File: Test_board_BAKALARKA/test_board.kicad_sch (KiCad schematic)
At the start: 6 parts, among them SW1 SW_SPST, SW2 SW_SPST, U2 ESP32-S3-WROOM-2

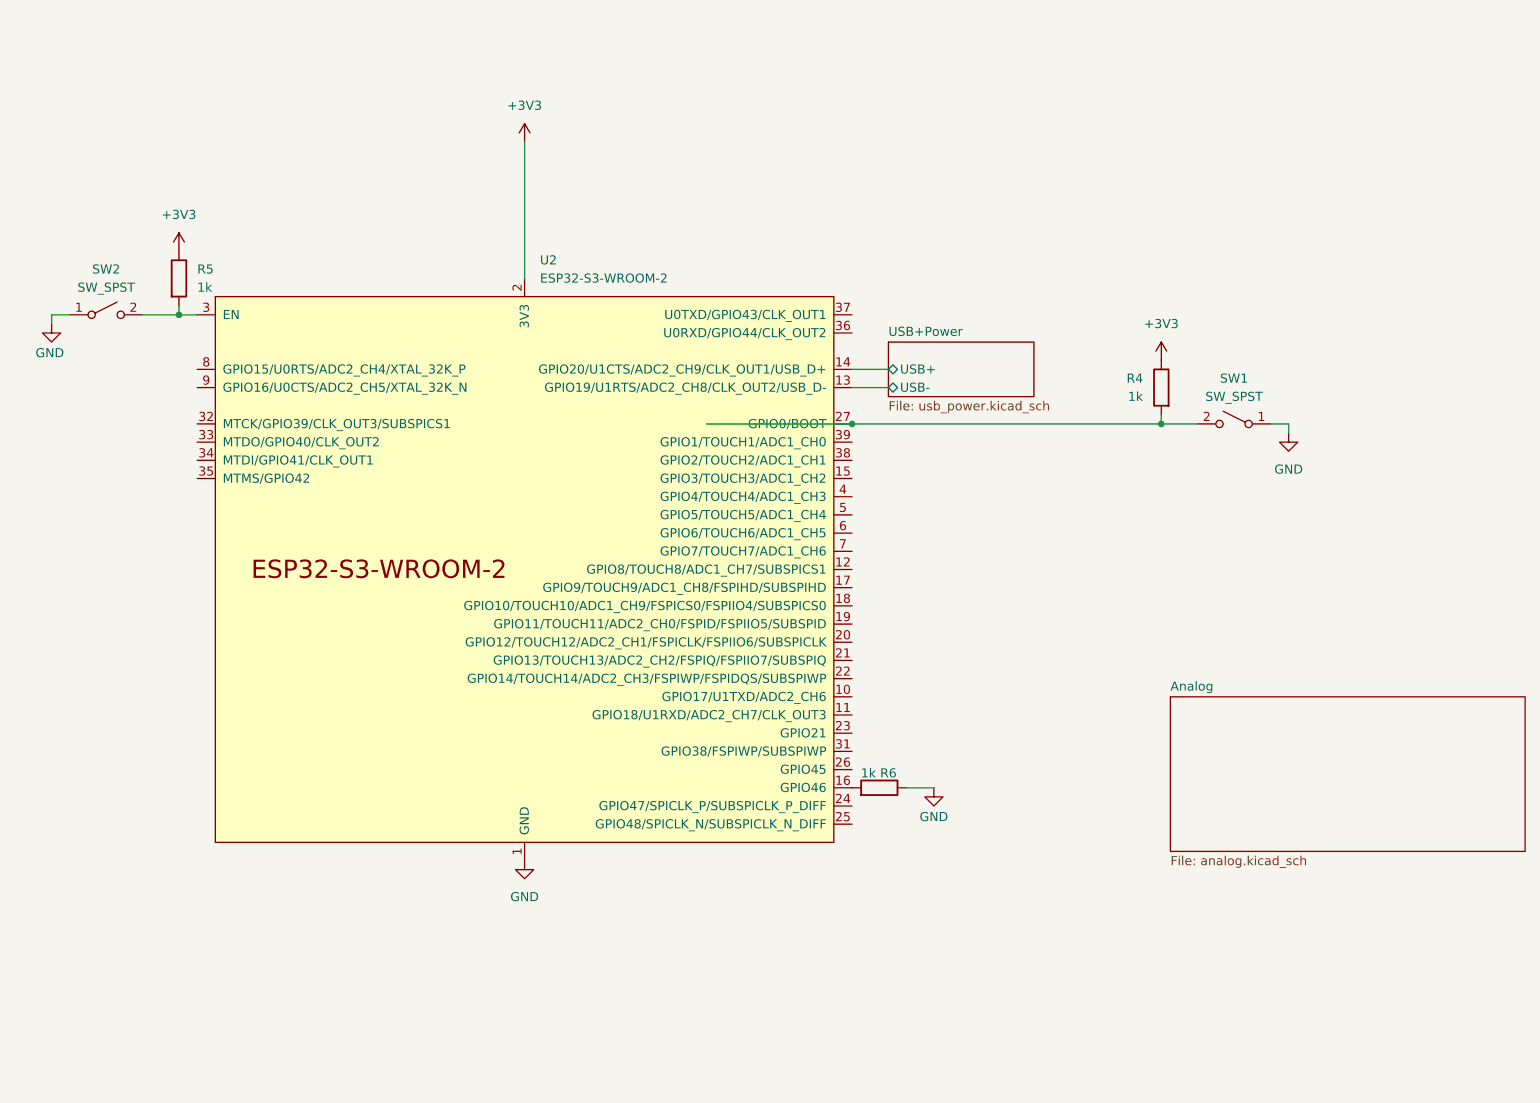
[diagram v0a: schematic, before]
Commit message: pridani textu peak detect, xor phase, signal source
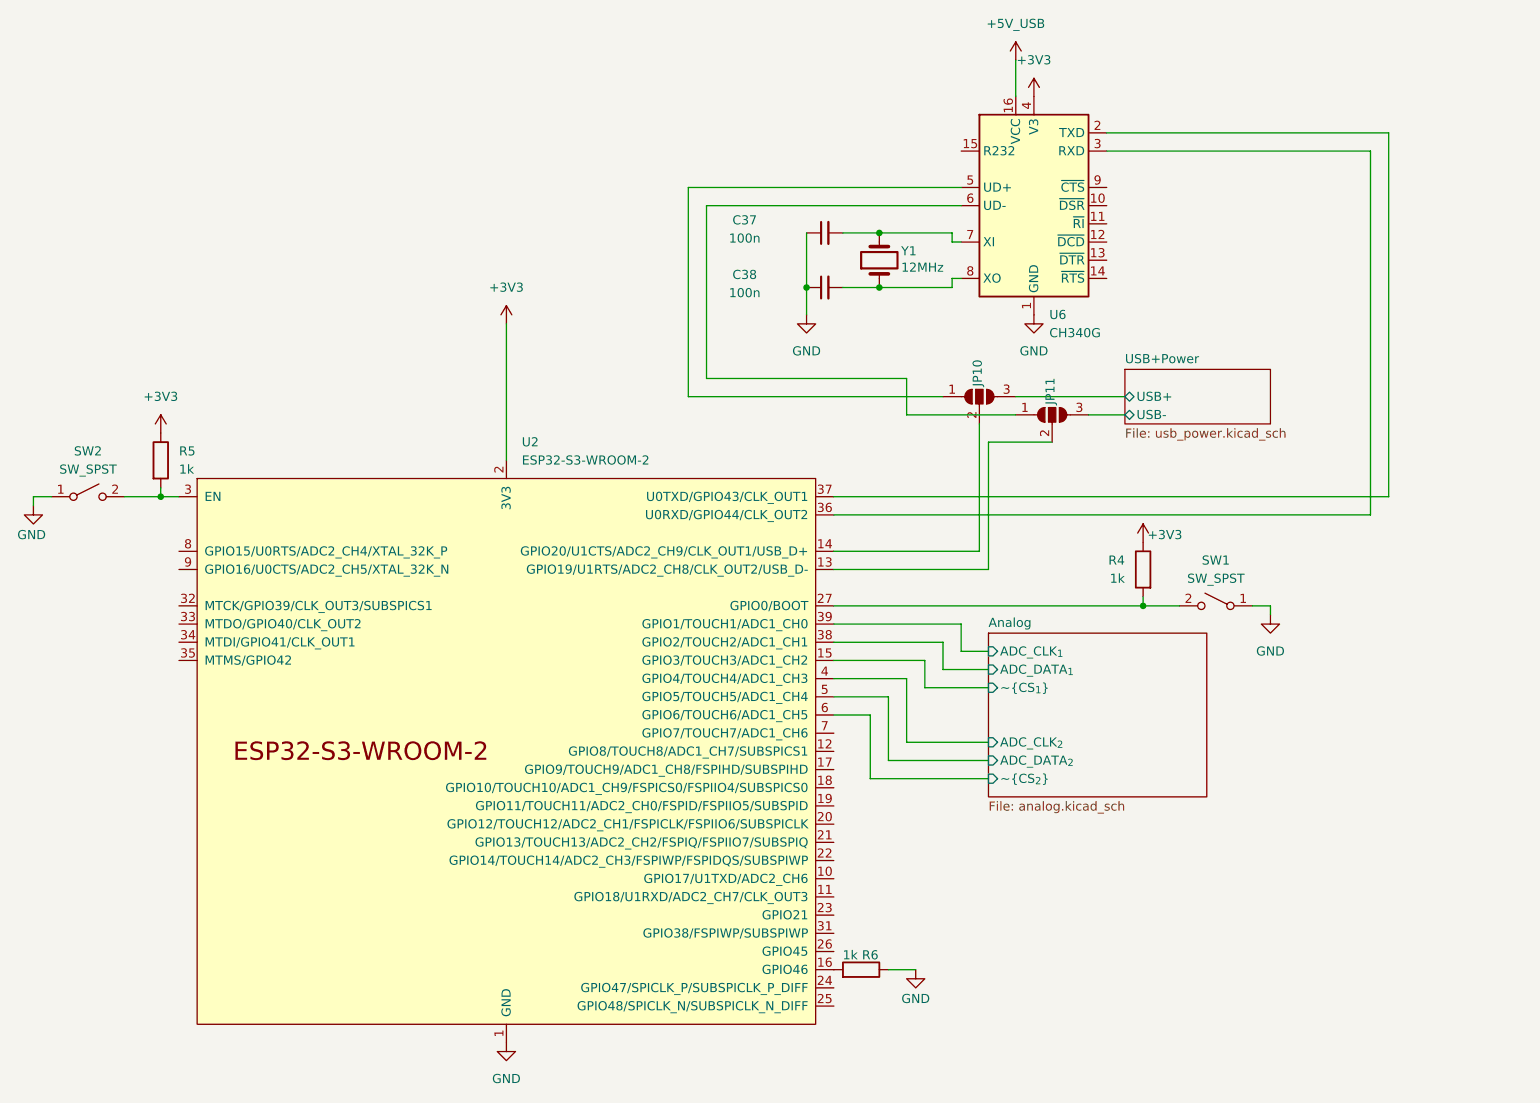
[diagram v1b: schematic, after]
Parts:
- added C37, C38: 100n, Capacitor_SMD:C_0603_1608Metric_Pad1.08x0.95mm_HandSolder, symbol Device:C_Small
- added JP10, JP11: SolderJumper_3_Open, Jumper:SolderJumper-3_P1.3mm_Open_RoundedPad1.0x1.5mm, symbol Jumper:SolderJumper_3_Open
- added U6: CH340G, Package_SO:SOIC-16_3.9x9.9mm_P1.27mm, symbol Interface_USB:CH340G
- added Y1: 12MHz, Crystal:Crystal_SMD_HC49-SD_HandSoldering, symbol Device:Crystal
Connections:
- net +3V3: now also U6.4 (V3)
- net GND: now also C37.1, C38.1, U6.1 (GND)
- net USB+Power/USB+: now also JP10.3 (B); no longer U2.14 (GPIO20/U1CTS/ADC2_CH9/CLK_OUT1/USB_D+)
- net USB+Power/USB-: now also JP11.3 (B); no longer U2.13 (GPIO19/U1RTS/ADC2_CH8/CLK_OUT2/USB_D-)
- net Analog/~{CS_{1}}: now reaches U2.15 (GPIO3/TOUCH3/ADC1_CH2)
- net at U2.36 (U0RXD/GPIO44/CLK_OUT2): now also U6.3 (RXD)
- net at U2.37 (U0TXD/GPIO43/CLK_OUT1): now also U6.2 (TXD)
- net Analog/ADC_DATA_{1}: now reaches U2.38 (GPIO2/TOUCH2/ADC1_CH1)
- net Analog/ADC_CLK_{1}: now reaches U2.39 (GPIO1/TOUCH1/ADC1_CH0)
- net Analog/ADC_CLK_{2}: now reaches U2.4 (GPIO4/TOUCH4/ADC1_CH3)
- net Analog/ADC_DATA_{2}: now reaches U2.5 (GPIO5/TOUCH5/ADC1_CH4)
- net Analog/~{CS_{2}}: now reaches U2.6 (GPIO6/TOUCH6/ADC1_CH5)
- new net: C37.2, U6.7 (XI), Y1.2
- new net: JP10.1 (A), U6.5 (UD+)
- new net: JP10.2 (C), U2.14 (GPIO20/U1CTS/ADC2_CH9/CLK_OUT1/USB_D+)
- new net: C38.2, U6.8 (XO), Y1.1
- new net: JP11.2 (C), U2.13 (GPIO19/U1RTS/ADC2_CH8/CLK_OUT2/USB_D-)
- new net: JP11.1 (A), U6.6 (UD-)
- new net +5V_USB: U6.16 (VCC)
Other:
- sheet Analog ports: added ADC_CLK_{1}, ADC_CLK_{2}, ADC_DATA_{1}, ADC_DATA_{2}, ~{CS_{1}}, ~{CS_{2}}; removed none
- moved on the sheet: R4, R5, R6, SW1, SW2, U2
